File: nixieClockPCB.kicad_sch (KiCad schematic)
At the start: 23 parts, among them M1 1364_HV, U1 74141, U10 WeMos_D1_mini, U2 74141, U3 74141, U4 74141, U5 74141, U6 74141, U7 74AHC595, U8 74AHC595, U9 74AHC595

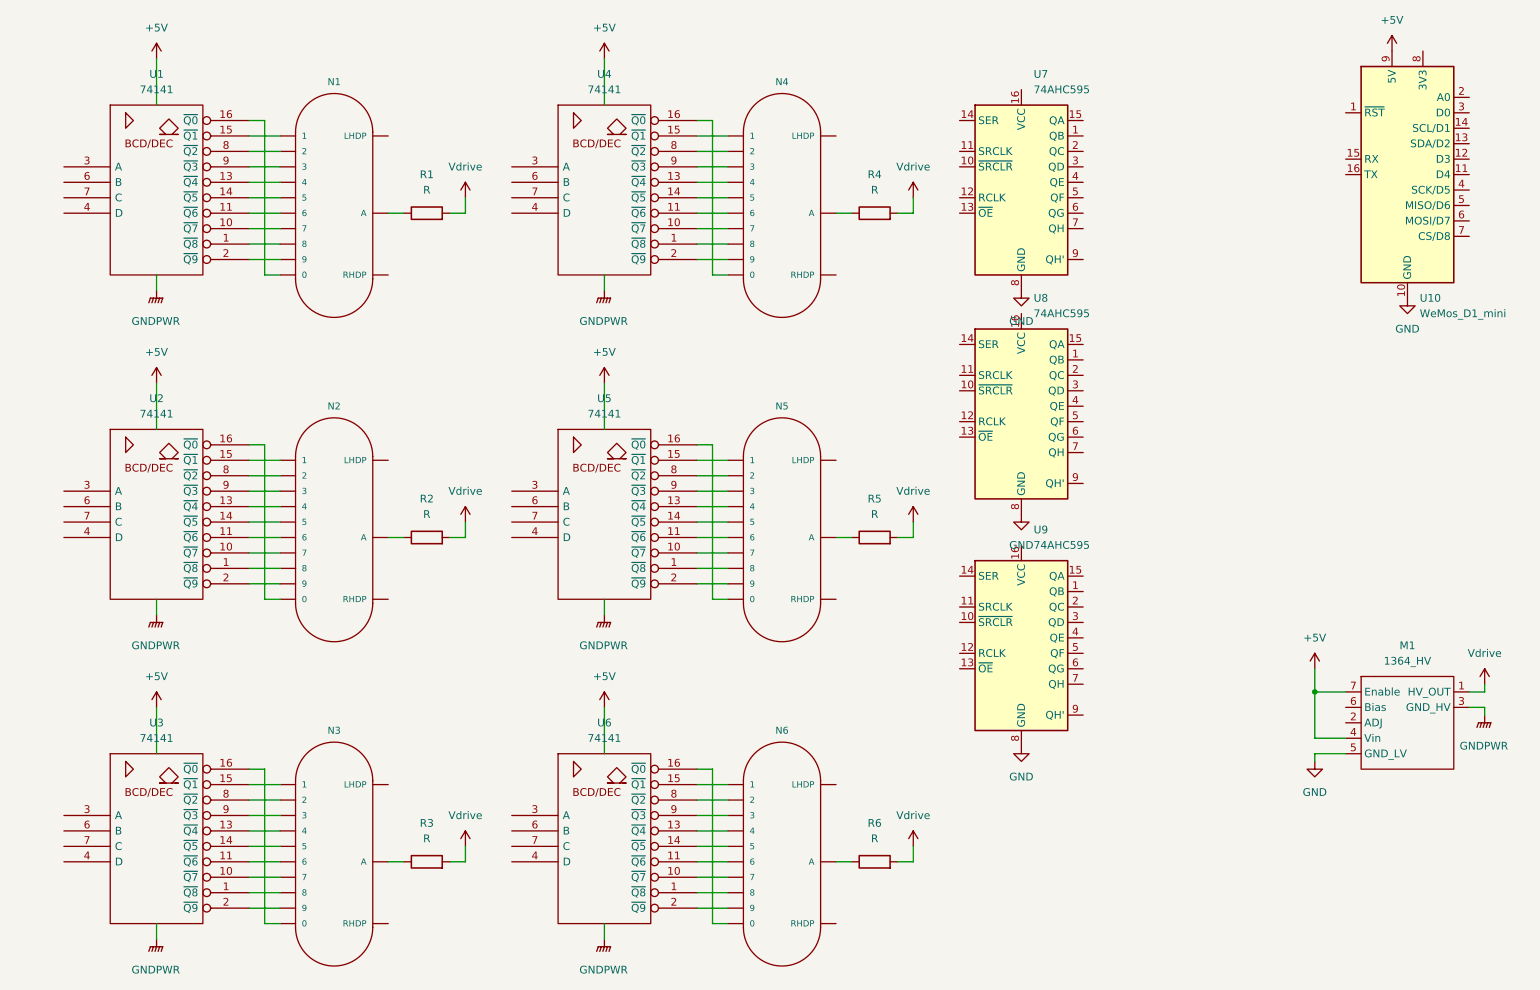
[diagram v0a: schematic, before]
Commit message: layout moving.
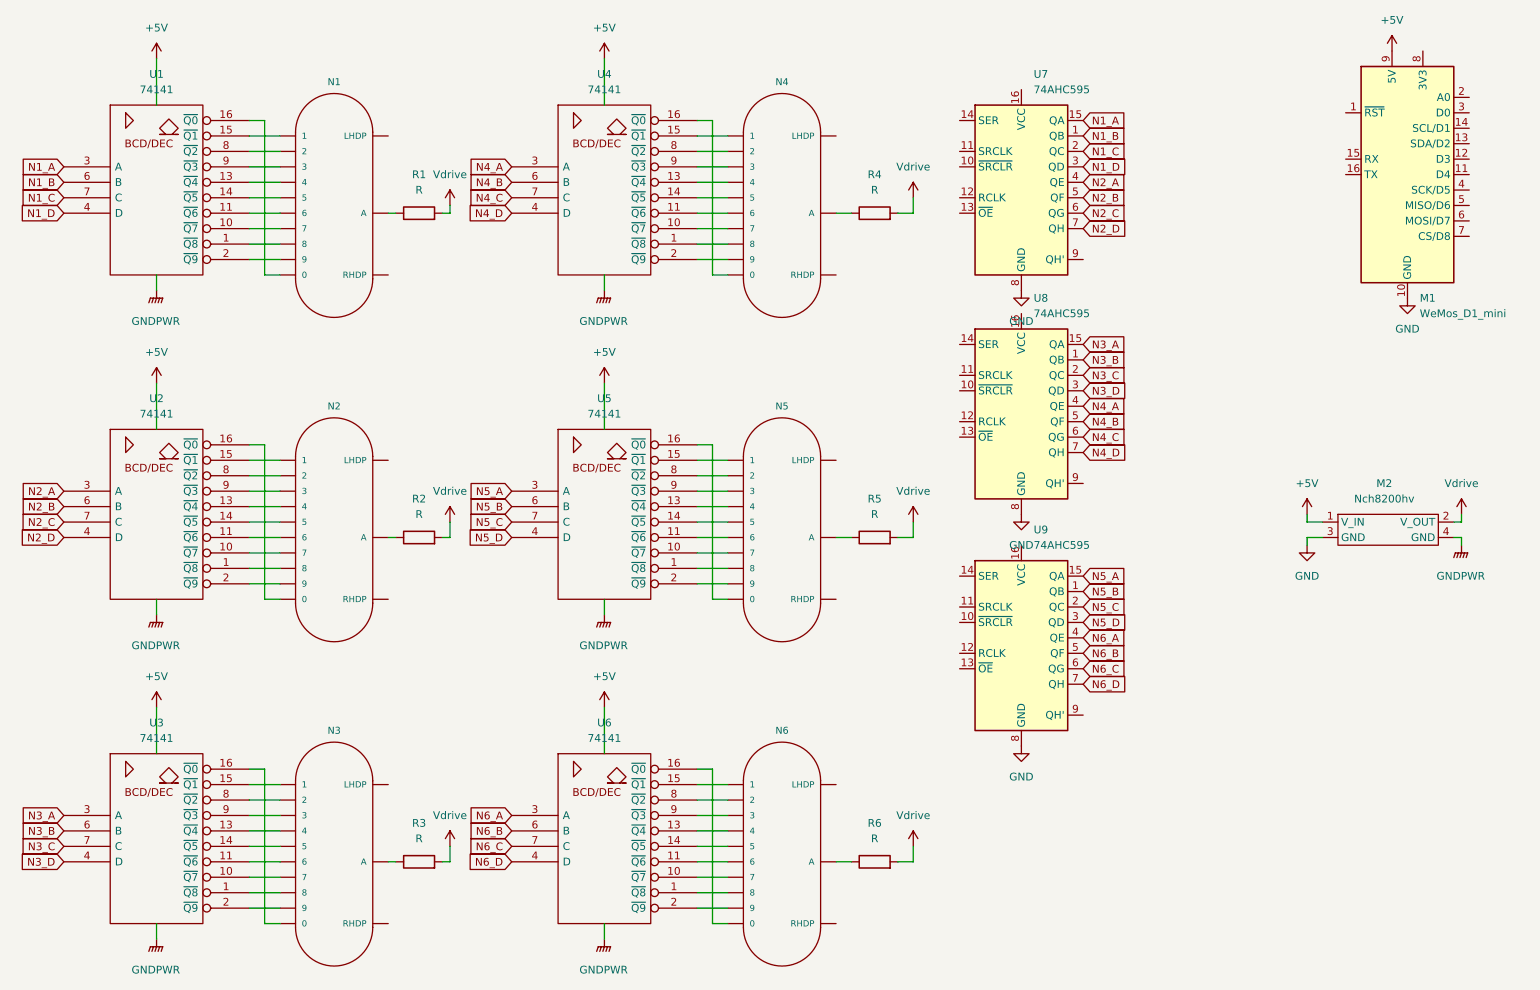
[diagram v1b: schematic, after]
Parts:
- removed M1: 1364_HV, Nixie_footprint_lib:1364_HV, symbol DCDC:1364_HV
- added M2: Nch8200hv, Nixie_footprint_lib:Nch8200hv, symbol nixieclock_project_lib:Nch8200hv
- U1, U2, U3, U4, U5, U6: footprint Package_DIP:DIP-16_W7.62mm_LongPads -> Package_DIP:DIP-16_W7.62mm
- U7, U8, U9: footprint Package_DIP:DIP-16_W7.62mm_LongPads -> nixiemisc:nixiemisc-SOIC16-5.3MM
- renumbered U10 to M1
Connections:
- net +5V: now also M2.1 (V_IN)
- net GND: now also M2.3 (GND), M2.4 (GND)
- net Vdrive: now also M2.2 (V_OUT)
- net N3_A: now reaches U3.3 (A)
- net N3_A: now also U8.15 (QA)
- net N3_D: now reaches U3.4 (D)
- net N3_D: now also U8.3 (QD)
- net N3_B: now reaches U3.6 (B)
- net N3_B: now also U8.1 (QB)
- net N3_C: now reaches U3.7 (C)
- net N3_C: now also U8.2 (QC)
- net N4_A: now reaches U8.4 (QE)
- net N4_A: now also U4.3 (A)
- net N4_B: now reaches U8.5 (QF)
- net N4_B: now also U4.6 (B)
- net N4_C: now reaches U8.6 (QG)
- net N4_C: now also U4.7 (C)
- net N4_D: now reaches U8.7 (QH)
- net N4_D: now also U4.4 (D)
- net N5_B: now reaches U9.1 (QB)
- net N5_B: now also U5.6 (B)
- net N5_A: now reaches U9.15 (QA)
- net N5_A: now also U5.3 (A)
- net N5_C: now reaches U9.2 (QC)
- net N5_C: now also U5.7 (C)
- net N5_D: now reaches U9.3 (QD)
- net N5_D: now also U5.4 (D)
- net N6_A: now reaches U9.4 (QE)
- net N6_A: now also U6.3 (A)
- net N6_B: now reaches U9.5 (QF)
- net N6_B: now also U6.6 (B)
- net N6_C: now reaches U9.6 (QG)
- net N6_C: now also U6.7 (C)
- net N6_D: now reaches U9.7 (QH)
- net N6_D: now also U6.4 (D)
- net N1_A: now reaches U1.3 (A)
- net N1_A: now also U7.15 (QA)
- net N1_D: now reaches U1.4 (D)
- net N1_D: now also U7.3 (QD)
- net N1_B: now reaches U1.6 (B)
- net N1_B: now also U7.1 (QB)
- net N1_C: now reaches U1.7 (C)
- net N1_C: now also U7.2 (QC)
- net N2_A: now reaches U7.4 (QE)
- net N2_A: now also U2.3 (A)
- net N2_B: now reaches U7.5 (QF)
- net N2_B: now also U2.6 (B)
- net N2_C: now reaches U7.6 (QG)
- net N2_C: now also U2.7 (C)
- net N2_D: now reaches U7.7 (QH)
- net N2_D: now also U2.4 (D)
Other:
- moved on the sheet: R1, R2, R3
